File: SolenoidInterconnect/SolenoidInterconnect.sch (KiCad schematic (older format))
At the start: 40 parts, among them J1 16PIN_IN, J10 Screw_Terminal_01x02, J11 Screw_Terminal_01x02, J12 Screw_Terminal_01x02, J13 Screw_Terminal_01x02, J14 Screw_Terminal_01x02, J15 Screw_Terminal_01x02, J16 Screw_Terminal_01x02, J17 Screw_Terminal_01x02, J18 Screw_Terminal_01x02, J19 Screw_Terminal_01x02, J2 16PIN_IN, J20 Screw_Terminal_01x02, J21 Screw_Terminal_01x02, J22 Screw_Terminal_01x02, J23 Screw_Terminal_01x02, J24 Screw_Terminal_01x02, J25 Screw_Terminal_01x02, J26 Screw_Terminal_01x02, J27 Screw_Terminal_01x02, J28 Screw_Terminal_01x02, J29 Screw_Terminal_01x02, J3 16PIN_IN, J30 Screw_Terminal_01x02, J31 Screw_Terminal_01x02, J32 Screw_Terminal_01x02, J33 Screw_Terminal_01x02, J34 Screw_Terminal_01x02, J35 Screw_Terminal_01x02, J36 Screw_Terminal_01x02, J37 16PIN_OUT, J38 16PIN_OUT, J39 16PIN_OUT, J4 16PIN_IN, J40 16PIN_OUT, J5 Screw_Terminal_01x02, J6 Screw_Terminal_01x02, J7 Screw_Terminal_01x02, J8 Screw_Terminal_01x02, J9 Screw_Terminal_01x02

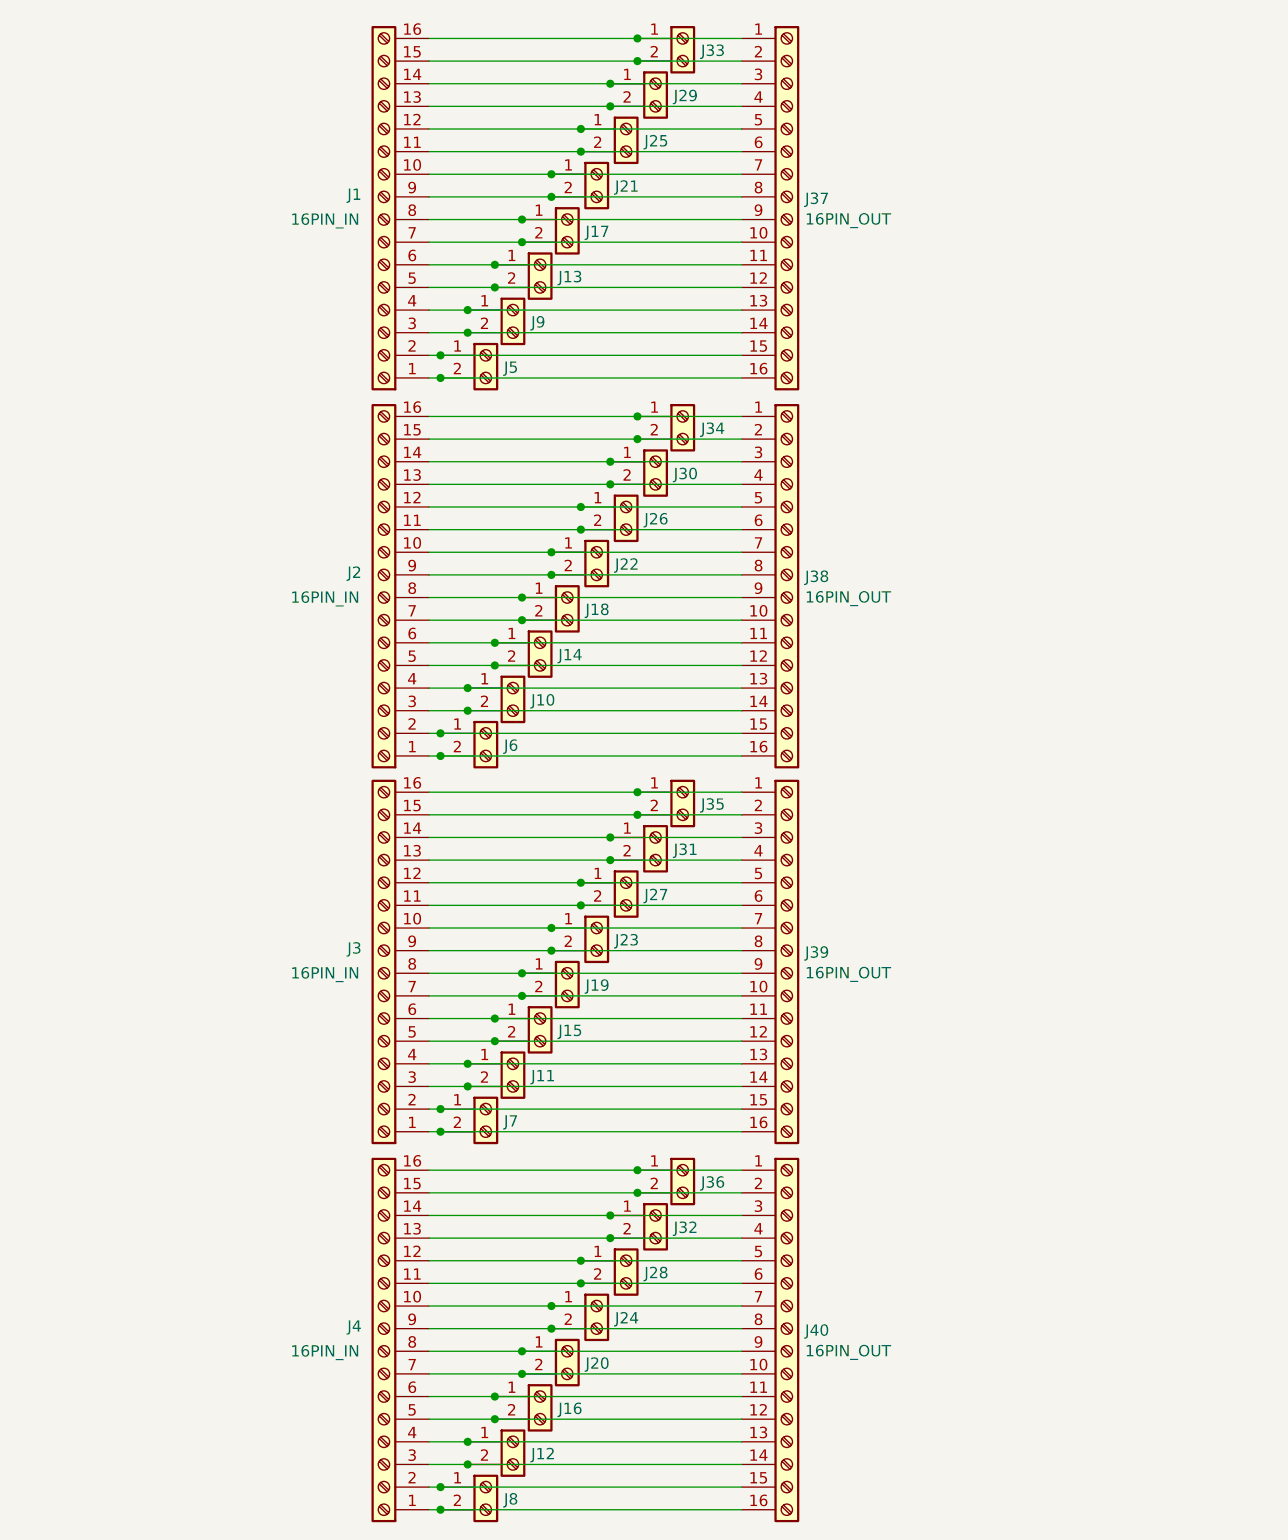
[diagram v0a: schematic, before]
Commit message: V1.0
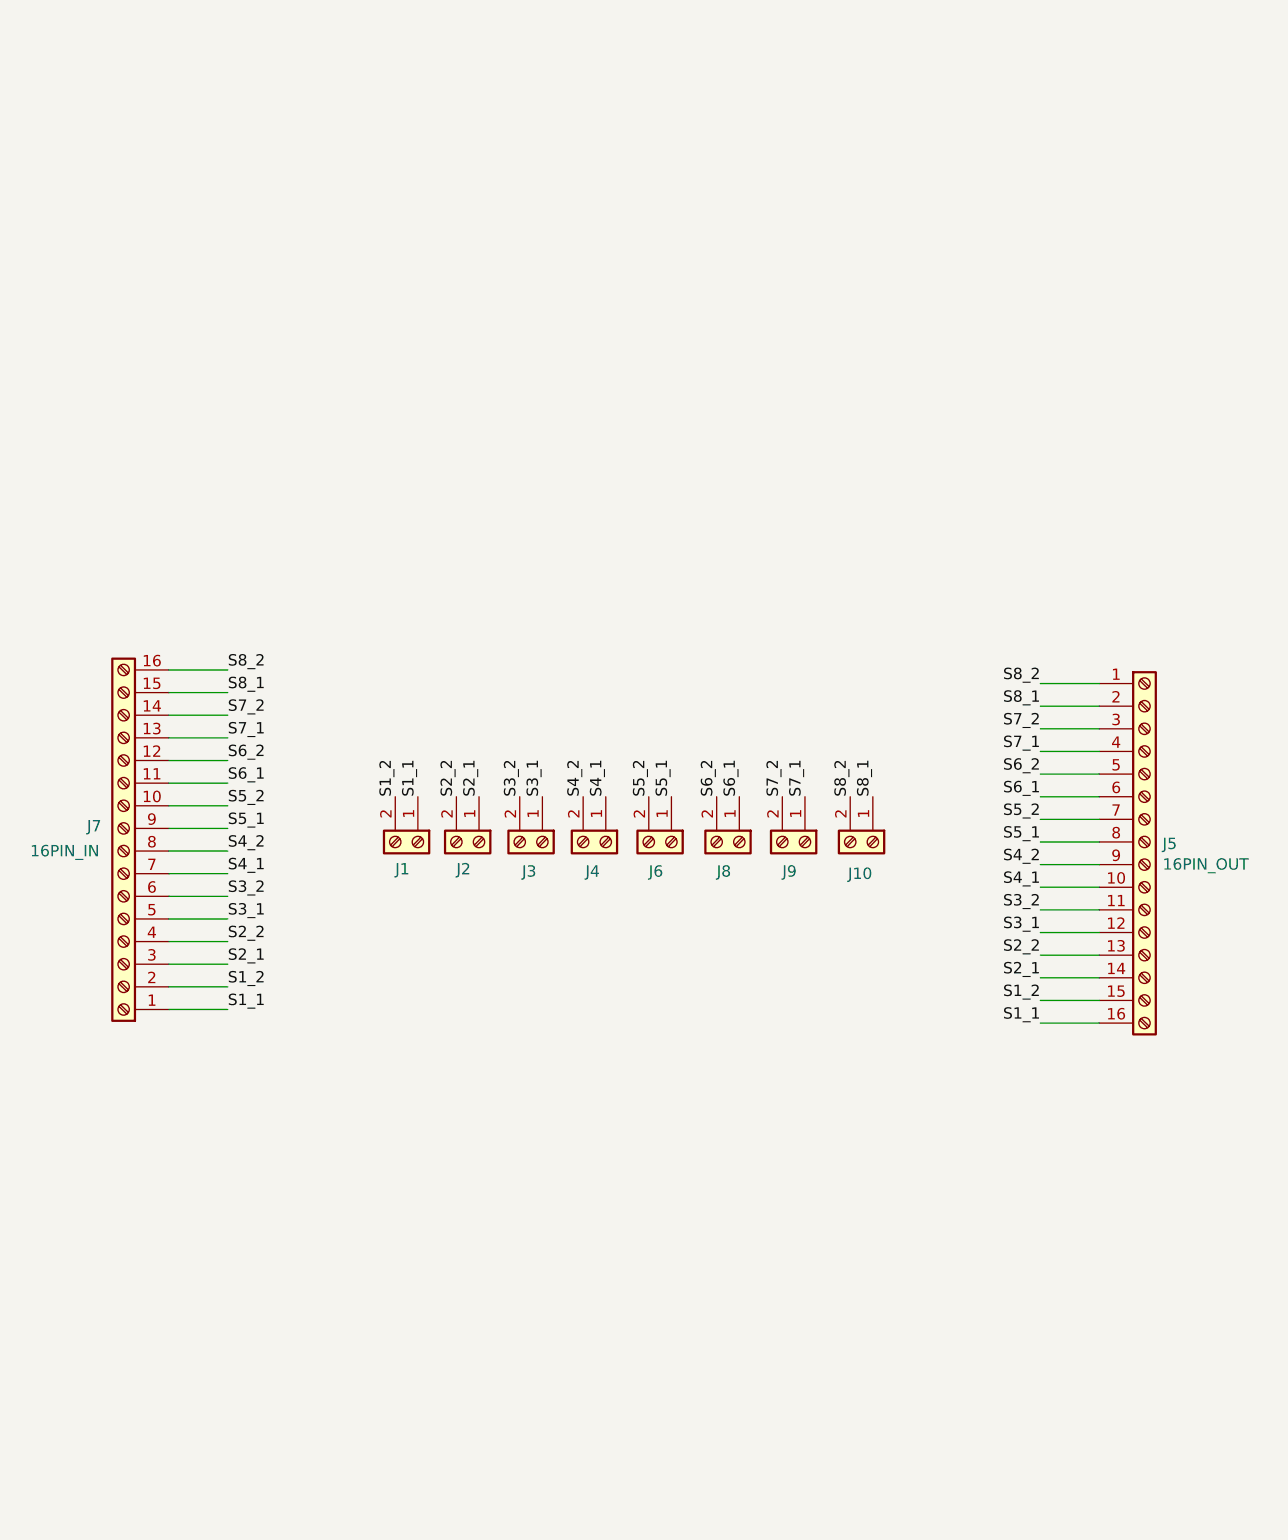
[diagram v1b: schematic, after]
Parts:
- removed J1, J2, J3, J4: 16PIN_IN, symbol Connector:Screw_Terminal_01x16
- removed J11, J12, J13, J14, J15, J16, J17, J18, J19, J20, J21, J22, J23, J24, J25, J26, J27, J28, J29, J30, J31, J32, J33, J34, J35, J36, J5, J7: Screw_Terminal_01x02, TerminalBlock_4Ucon:TerminalBlock_4Ucon_1x02_P3.50mm_Vertical, symbol Connector:Screw_Terminal_01x02
- removed J37, J38, J39, J40: 16PIN_OUT, symbol Connector:Screw_Terminal_01x16
- added J1, J2, J3, J4: Screw_Terminal_01x02, LocalLib:2PIN_CH, symbol Connector:Screw_Terminal_01x02
- added J5: 16PIN_OUT, LocalLib:16PIN_CH, symbol Connector:Screw_Terminal_01x16
- added J7: 16PIN_IN, LocalLib:16PIN_CH, symbol Connector:Screw_Terminal_01x16
- J10, J6, J8, J9: footprint TerminalBlock_4Ucon:TerminalBlock_4Ucon_1x02_P3.50mm_Vertical -> LocalLib:2PIN_CH
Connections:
- net S7_1: now reaches J9.1 (Pin_1)
- net S7_1: now also J5.4 (Pin_4), J7.13 (Pin_13)
- net S7_2: now reaches J9.2 (Pin_2)
- net S7_2: now also J5.3 (Pin_3), J7.14 (Pin_14)
- net S5_1: now reaches J6.1 (Pin_1)
- net S5_1: now also J5.8 (Pin_8), J7.9 (Pin_9)
- net S5_2: now reaches J6.2 (Pin_2)
- net S5_2: now also J5.7 (Pin_7), J7.10 (Pin_10)
- net S8_1: now reaches J10.1 (Pin_1)
- net S8_1: now also J5.2 (Pin_2), J7.15 (Pin_15)
- net S8_2: now reaches J10.2 (Pin_2)
- net S8_2: now also J5.1 (Pin_1), J7.16 (Pin_16)
- net S6_1: now reaches J8.1 (Pin_1)
- net S6_1: now also J5.6 (Pin_6), J7.11 (Pin_11)
- net S6_2: now reaches J8.2 (Pin_2)
- net S6_2: now also J5.5 (Pin_5), J7.12 (Pin_12)
- new net S1_1: J1.1 (Pin_1), J5.16 (Pin_16), J7.1 (Pin_1)
- new net S1_2: J1.2 (Pin_2), J5.15 (Pin_15), J7.2 (Pin_2)
- new net S2_1: J2.1 (Pin_1), J5.14 (Pin_14), J7.3 (Pin_3)
- new net S2_2: J2.2 (Pin_2), J5.13 (Pin_13), J7.4 (Pin_4)
- new net S3_1: J3.1 (Pin_1), J5.12 (Pin_12), J7.5 (Pin_5)
- new net S3_2: J3.2 (Pin_2), J5.11 (Pin_11), J7.6 (Pin_6)
- new net S4_1: J4.1 (Pin_1), J5.10 (Pin_10), J7.7 (Pin_7)
- new net S4_2: J4.2 (Pin_2), J5.9 (Pin_9), J7.8 (Pin_8)
